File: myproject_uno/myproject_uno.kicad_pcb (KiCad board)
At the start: 2 copper layers, 68.6 x 53.3 mm, 10 parts, among them P1 Power, P2 Analog, P3 Digital, P4 Digital, P5 CONN_01X01, P6 CONN_01X01, P7 CONN_01X01, P8 CONN_01X01

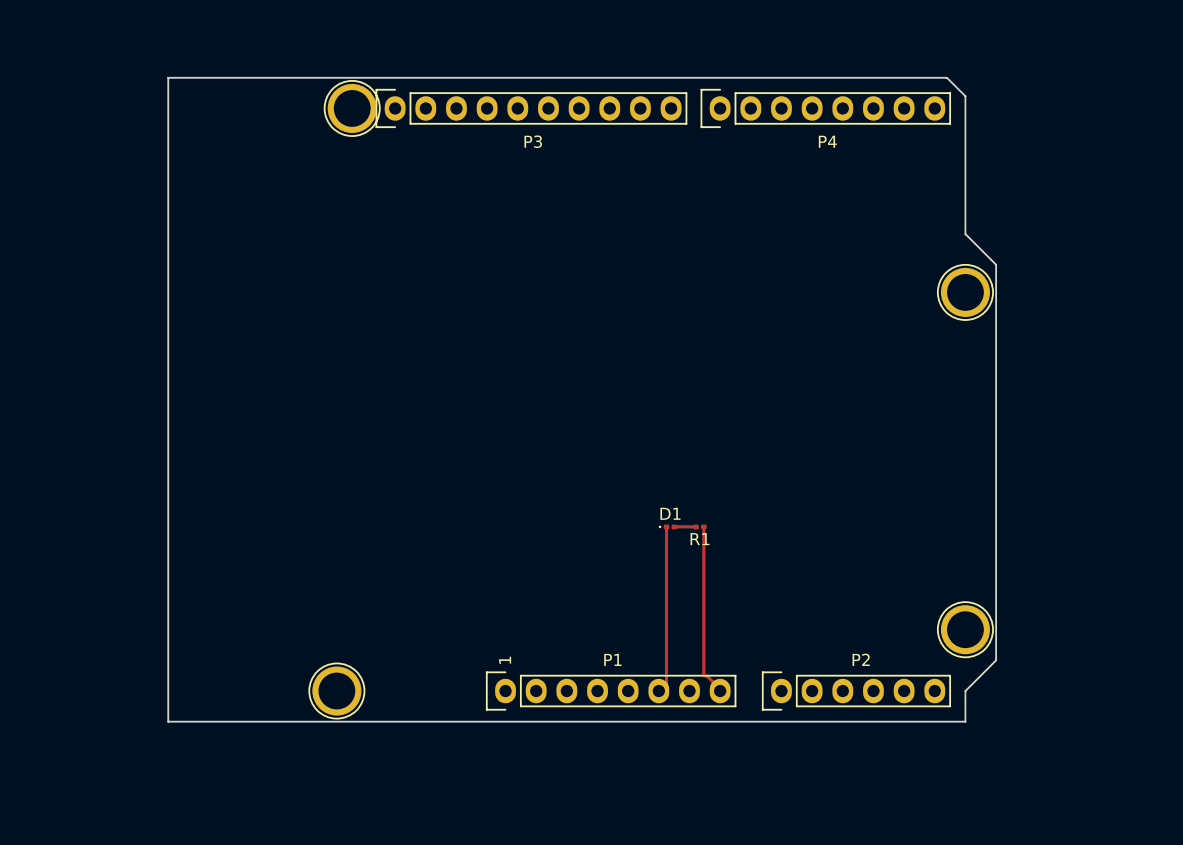
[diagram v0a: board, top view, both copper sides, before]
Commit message: pcb almost designed
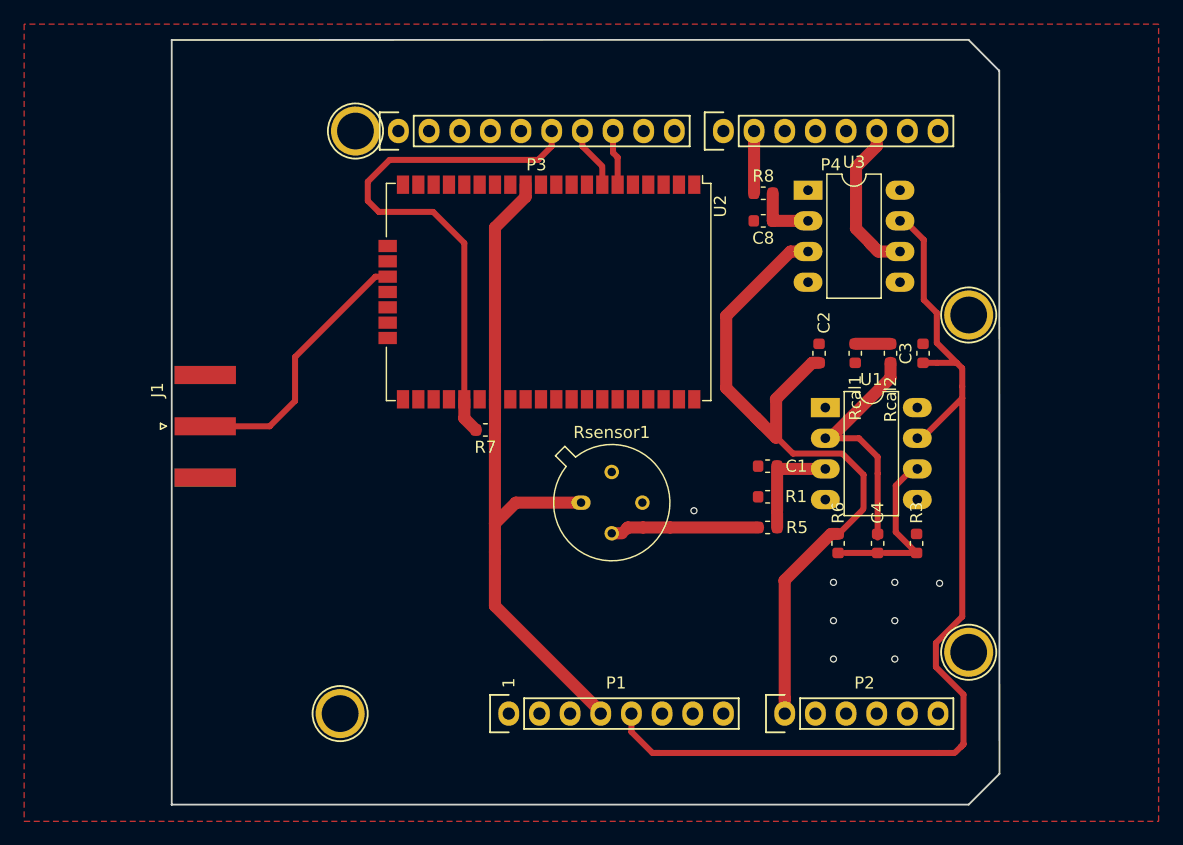
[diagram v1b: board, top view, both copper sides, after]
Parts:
- removed D1: LED, LED_SMD:LED_0201_0603Metric
- added C1: 100n, Capacitor_SMD:C_0603_1608Metric, F.Cu at (160.6, 105.2)
- added C2: 100n, Capacitor_SMD:C_0603_1608Metric, F.Cu at (164.9, 95.8)
- added C3: 100n, Capacitor_SMD:C_0603_1608Metric, F.Cu at (173.5, 95.8)
- added C4: 1u, Capacitor_SMD:C_0603_1608Metric, F.Cu at (169.8, 111.6)
- added C8: 0,1u, Capacitor_SMD:C_0603_1608Metric, F.Cu at (160.3, 84.9)
- added J1: Conn_Coaxial, Connector_Coaxial:SMA_Amphenol_132289_EdgeMount, F.Cu at (114.1, 101.9)
- added R3: 100K, Resistor_SMD:R_0603_1608Metric, F.Cu at (173.0, 111.6)
- added R5: 100K, Resistor_SMD:R_0603_1608Metric, F.Cu at (160.6, 110.3)
- added R6: 1K, Resistor_SMD:R_0603_1608Metric, F.Cu at (166.5, 111.6)
- added R7: 10K, Resistor_SMD:R_0603_1608Metric, F.Cu at (137.3, 102.2)
- added R8: 100K, Resistor_SMD:R_0603_1608Metric, F.Cu at (160.3, 82.6)
- added Rcal1: R, Resistor_SMD:R_0603_1608Metric, F.Cu at (167.9, 95.8)
- added Rcal2: R, Resistor_SMD:R_0603_1608Metric, F.Cu at (170.8, 95.8)
- added Rsensor1: R, Package_TO_SOT_THT:TO-5-4, F.Cu at (145.2, 108.2)
- added U1: LTC1050, Package_DIP:DIP-8_W7.62mm_LongPads, F.Cu at (165.4, 100.3)
- added U2: RN2483, RF_Module:RN2483, F.Cu at (142.5, 90.8)
- added U3: LTC1050, Package_DIP:DIP-8_W7.62mm_LongPads, F.Cu at (164.0, 82.3)
- R1: value R -> 100K; footprint Resistor_SMD:R_0201_0603Metric -> Resistor_SMD:R_0603_1608Metric
- moved R1 6.14 mm to (160.6, 107.7)
- moved P1 1.89 mm to (139.2, 125.7)
- moved P4 1.89 mm to (157.0, 77.4)
- moved P2 1.89 mm to (162.1, 125.7)
- moved P3 1.89 mm to (130.1, 77.4)
- moved P5 1.89 mm to (125.2, 125.7)
- moved P6 1.89 mm to (177.3, 120.6)
- moved P7 1.89 mm to (126.5, 77.4)
- moved P8 1.89 mm to (177.3, 92.7)
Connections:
- P2 pad 1: /A0 -> ANxArduino
- P3 pad 6: /12(MISO) -> !RST
- P3 pad 7: /11(**/MOSI) -> RX
- P3 pad 8: /10(**/SS) -> TX
- P4 pad 2: /6(**) -> Vref
- P4 pad 6: /2 -> INT
- R1 pad 1: /Vin -> Net-(C1-Pad1)
- R1 pad 2: Net-(D1-Pad2) -> GND
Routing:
- net +5V: track 0.00 -> 87.1 mm
- net ANxArduino: track 0.00 -> 61.3 mm
- net +3V3: track 0.00 -> 57.7 mm
- net !RST: track 0.00 -> 44.6 mm
- net Net-(J1-Pad1): track 0.00 -> 22.4 mm
- net Net-(C4-Pad1): track 0.00 -> 21.3 mm
- net Net-(C4-Pad2): track 0.00 -> 16.1 mm
- net /Vin: track 14.2 -> 0.15 mm
- net INT: track 0.00 -> 14.0 mm
- net GND: track 13.9 -> 0.00 mm, vias 0 -> 8
- net Net-(R5-Pad1): track 0.00 -> 12.3 mm
- net Net-(C1-Pad1): track 0.00 -> 9.97 mm
- net Net-(C8-Pad1): track 0.00 -> 5.21 mm
- net Vref: track 0.00 -> 5.17 mm
- net RX: track 0.00 -> 4.61 mm
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- added copper zone on F.Cu, net GND
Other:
- board size 68.6 x 53.3 mm -> 68.6 x 63.4 mm
